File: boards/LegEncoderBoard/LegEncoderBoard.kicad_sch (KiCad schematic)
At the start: 38 parts, among them J1 Conn_01x05, Q1 MMBT3904, Q2 MMBT3904, Q3 MMBT3904, U1 AS5047P-ATST, U2 SN74LVC3G17DCTR

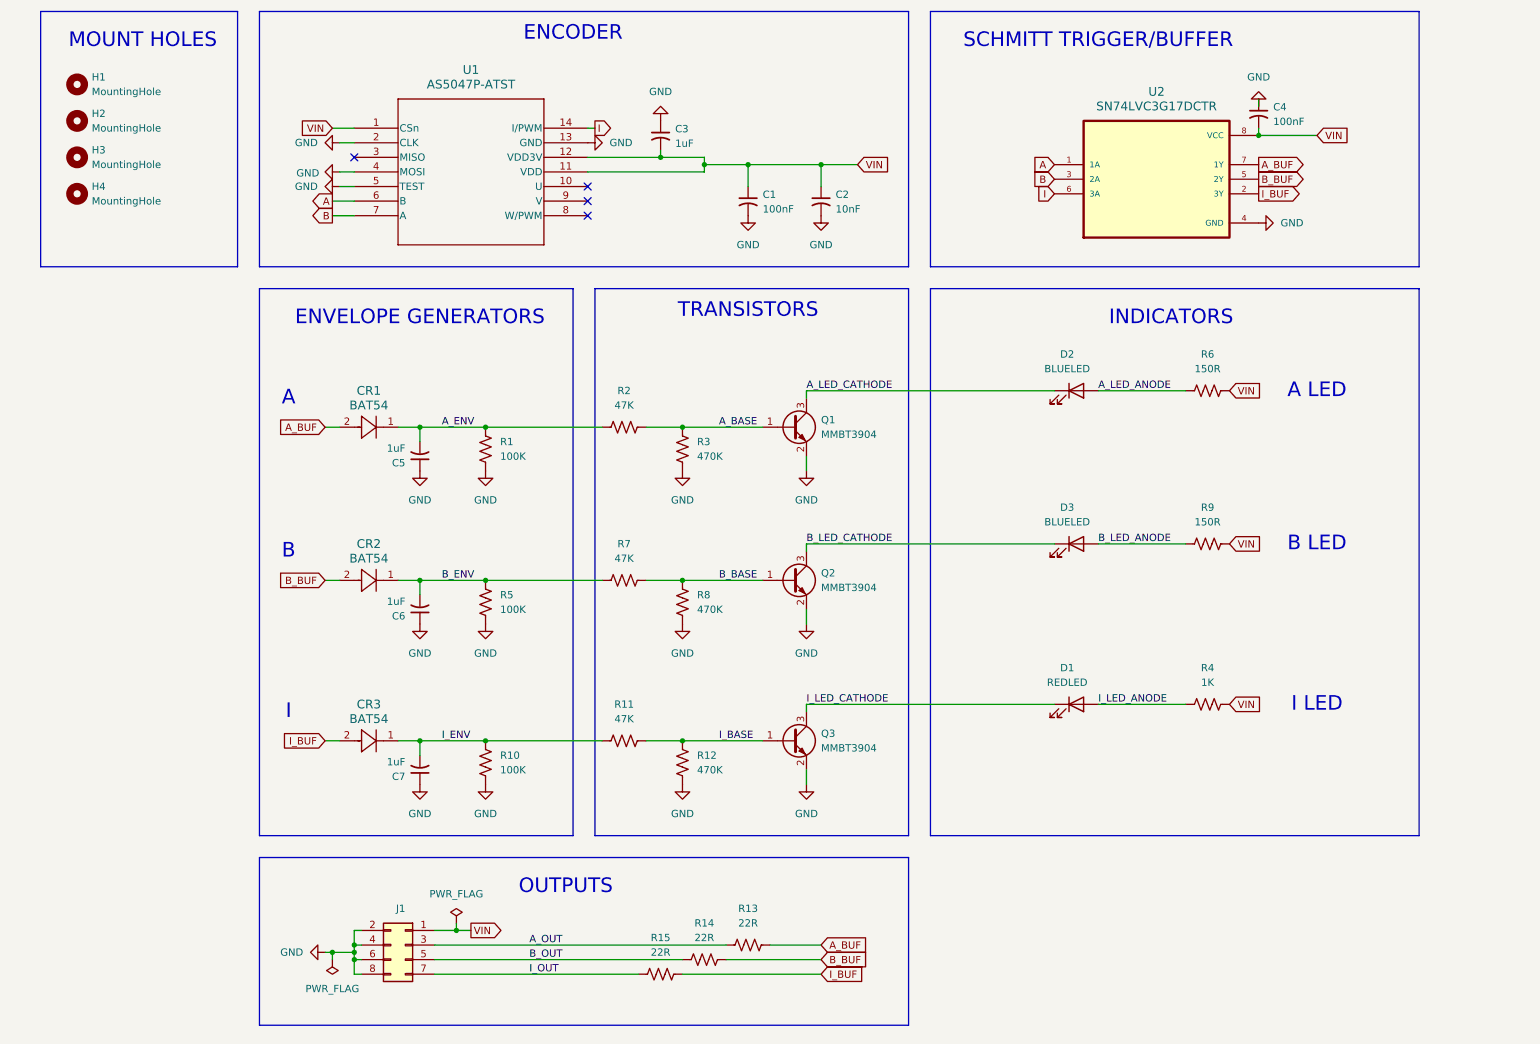
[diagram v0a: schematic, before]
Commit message: Finalize leg encoder board iteration
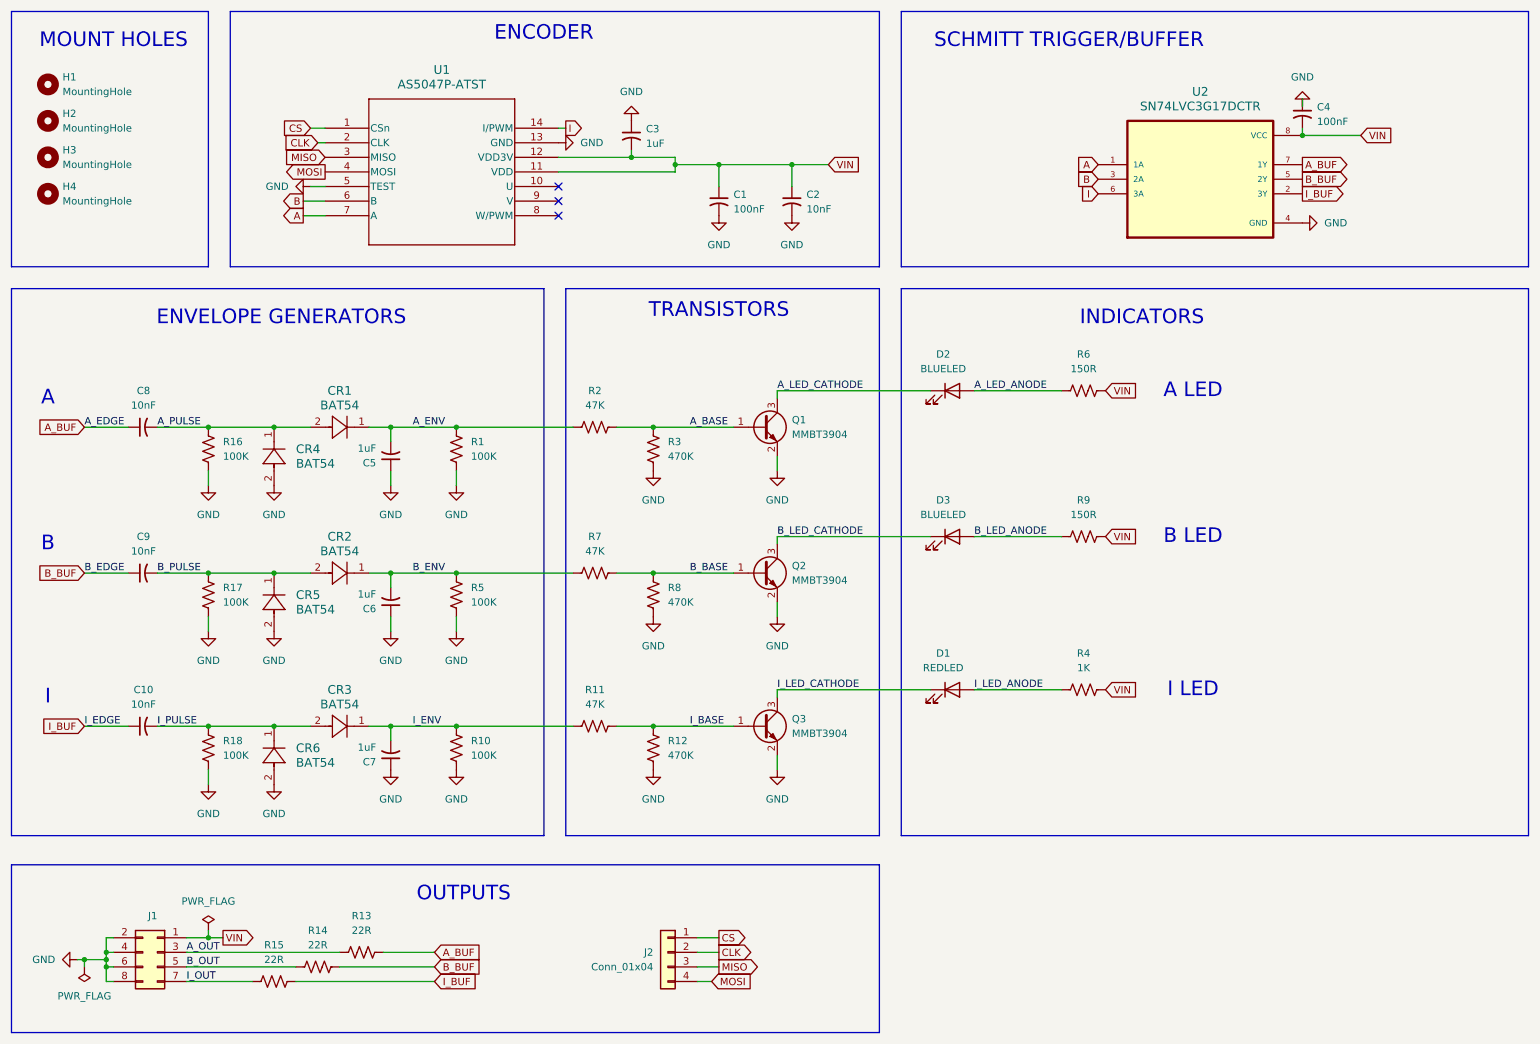
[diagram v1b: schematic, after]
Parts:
- added C10, C8, C9: 10nF, Capacitor10nF:GRM1885C1H103JA01D, symbol Device:C_Small_US
- added CR4, CR5, CR6: BAT54, EnvelopeDiode:BAT54WS-7-F, symbol EnvelopeDiode:BAT54WS-7-F
- added J2: Conn_01x04, Connector_JST:JST_XH_B4B-XH-A_1x04_P2.50mm_Vertical, symbol Connector_Generic:Conn_01x04
- added R16, R17, R18: 100K, Resistor100K:CRCW0603100KFKEA, symbol Device:R_US
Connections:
- net A: now also U1.7 (A); no longer U1.6 (B)
- net A_BUF: now also C8.1; no longer CR1.2
- net B: now also U1.6 (B); no longer U1.7 (A)
- net B_BUF: now also C9.1; no longer CR2.2
- net GND: now also CR4.2, CR5.2, CR6.2, R16.2, R17.2, R18.2; no longer U1.2 (CLK), U1.4 (MOSI)
- net I_BUF: now also C10.1; no longer CR3.2
- net VIN: no longer U1.1 (CSn)
- net MISO: now reaches U1.3 (MISO)
- net MISO: now also J2.3 (Pin_3)
- new net A_PULSE: C8.2, CR1.2, CR4.1, R16.1
- new net B_PULSE: C9.2, CR2.2, CR5.1, R17.1
- new net CLK: J2.2 (Pin_2), U1.2 (CLK)
- new net CS: J2.1 (Pin_1), U1.1 (CSn)
- new net I_PULSE: C10.2, CR3.2, CR6.1, R18.1
- new net MOSI: J2.4 (Pin_4), U1.4 (MOSI)
- no-connect marks 4 -> 3
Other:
- moved on the sheet: C1, C2, C3, C4, C5, C6, C7, CR1, CR2, CR3, D1, D2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
